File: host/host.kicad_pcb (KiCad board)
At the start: 4 copper layers, 22 x 44 mm, 31 parts, among them J1 Conn_01x02, J2 USB_A, J3 Conn_01x05, J4 Conn_01x05, SW1 SW_SPDT, SW2 SW_SPST, U1 AP2127N-3.3, U2 USBLC6-2SC6, U3 STM32F401RCT6, Y1 8M

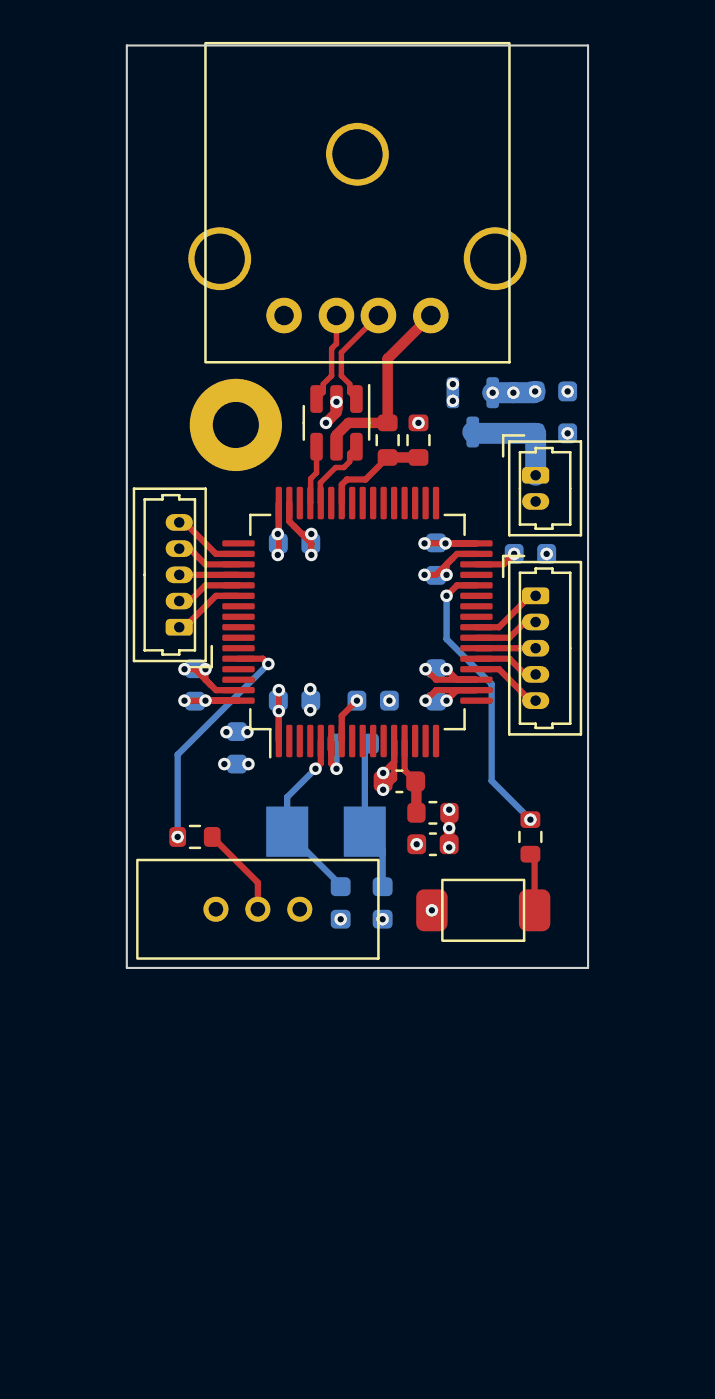
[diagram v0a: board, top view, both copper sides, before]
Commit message: power v1, updated host to v2
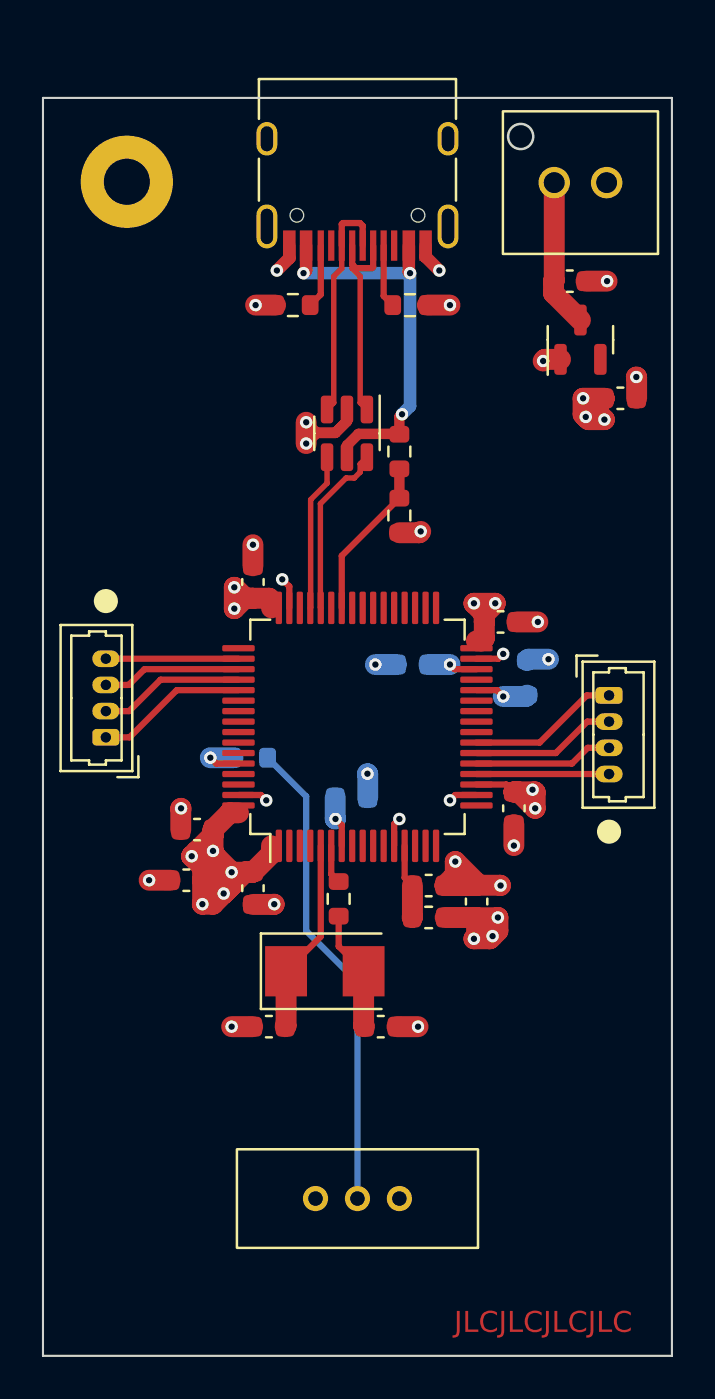
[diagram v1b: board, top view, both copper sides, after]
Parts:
- removed SW2: SW_SPST, KLIB:ALPS_SKRKAEE020
- added R6: 5.1K, Resistor_SMD:R_0603_1608Metric, F.Cu at (127.5, 79.9)
- added R7: 5.1K, Resistor_SMD:R_0603_1608Metric, F.Cu at (121.9, 79.9)
- C1, C11, C12, C2, C3, C4, C5, C6, C7, C8, U1, Y1: moved to F.Cu
- J1: footprint Connector_Molex:Molex_PicoBlade_53047-0210_1x02_P1.25mm_Vertical -> klib:MOLEX_533750210-Mini-Lock-2Pin-Through-Hole
- J2: value USB_A -> USB_C_Receptacle_USB2.0; footprint KLIB:JST_UBA-4R-D14T-4D -> Connector_USB:USB_C_Receptacle_HRO_TYPE-C-31-M-12
- J3, J4: value Conn_01x05 -> Conn_01x04; footprint Connector_Molex:Molex_PicoBlade_53047-0510_1x05_P1.25mm_Vertical -> Connector_Molex:Molex_PicoBlade_53047-0410_1x04_P1.25mm_Vertical
- R1: renamed from R3; moved to F.Cu
- R2: renamed from R4; moved to B.Cu
- R3: renamed from R5; moved to B.Cu
- R4: renamed from R1; value 33K -> 48K
- R5: renamed from R2; value 82K -> 72K
- SW1: footprint KLIB:ALPS_SSSS912000 -> klib:ALPS_SSSS912000
- moved SW1 14.6 mm to (125.0, 122.5)
- moved J1 14.1 mm to (135.6, 74.0), turned to 180 degrees
- moved H1 12.7 mm to (114.0, 74.0)
- moved C4 9.16 mm to (120.0, 107.7), turned to -90 degrees
- moved C13 7.71 mm to (127.6, 97.0), turned to 180 degrees
- moved R3 7.59 mm to (133.1, 97.7), turned to -90 degrees
- moved R1 7.44 mm to (124.1, 108.2), turned to -90 degrees
- moved C1 7.31 mm to (135.1, 78.7)
- moved C5 6.96 mm to (132.5, 103.9)
- moved C8 6.90 mm to (117.3, 104.9), turned to 180 degrees
- moved C11 6.82 mm to (120.8, 114.3), turned to 180 degrees
- moved C3 6.76 mm to (116.8, 107.3), turned to 180 degrees
- moved Y1 6.66 mm to (123.4, 111.7)
- moved J3 6.31 mm to (113.0, 100.5)
- moved U1 6.20 mm to (135.6, 81.5), turned to 90 degrees
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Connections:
- J1 pad 1: 5V -> GND
- J1 pad 2: GND -> 5V
- J3 pad 1: MSC_L -> MOSI_L
- J3 pad 2: MOSI_L -> MISO_L
- J3 pad 3: MISO_L -> SCK_L
- J3 pad 4: SCK_L -> NSS_L
- J4 pad 1: MSC_R -> MOSI_R
- J4 pad 2: MOSI_R -> MISO_R
- J4 pad 3: MISO_R -> SCK_R
- J4 pad 4: SCK_R -> NSS_R
- R3 pad 1: Net-(R5-Pad1) -> GND
- R4 pad 1: RAW_USB_VBUS -> USB_VBUS
- R4 pad 2: USB_VBUS -> USB_VBUS_SIG
- R5 pad 1: USB_VBUS -> USB_VBUS_SIG
- U2 pad 1: RAW_USB_D- -> USB_RAW_D-
- U2 pad 3: RAW_USB_D+ -> USB_RAW_D+
- U2 pad 5: RAW_USB_VBUS -> USB_VBUS
- U3 pad 24: MSC_R -> unconnected-(U3-Pad24)
- U3 pad 42: USB_VBUS -> USB_VBUS_SIG
- U3 pad 54: MSC_L -> unconnected-(U3-Pad54)
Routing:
- net Net-(R2-Pad1): track 4.35 -> 22.8 mm
- net 3V3: track 29.9 -> 44.4 mm, vias 18 -> 17
- net USB_VBUS: track 5.07 -> 19.0 mm, vias 0 -> 3
- net BOOT1: track 14.0 -> 2.57 mm, vias 2 -> 1
- net GND: track 27.8 -> 39.1 mm, vias 27 -> 28
- net USB_RAW_D+: track 0.00 -> 11.2 mm
- net USB_RAW_D-: track 0.00 -> 11.1 mm
- net RAW_USB_VBUS: track 9.21 -> 0.00 mm
- net BOOT0: track 11.6 -> 2.54 mm, vias 2 -> 1
- net USB_VBUS_SIG: track 0.00 -> 7.77 mm
- net RAW_USB_D-: track 5.01 -> 0.00 mm
- net USB_D-: track 3.64 -> 8.34 mm
- net USB_D+: track 2.81 -> 7.52 mm
- net RAW_USB_D+: track 4.38 -> 0.00 mm
- net MOSI_R: track 3.14 -> 7.26 mm
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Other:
- board size 22 x 44 mm -> 30 x 60 mm
- board text added: "JLCJLCJLCJLC"
